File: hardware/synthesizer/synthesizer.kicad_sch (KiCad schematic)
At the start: 5 parts, among them J2 Input 2, J3 Input 1, J4 Output 1, J5 Output 2, J7 RJ45_Abracon_ARJP11A-MASA-B-A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

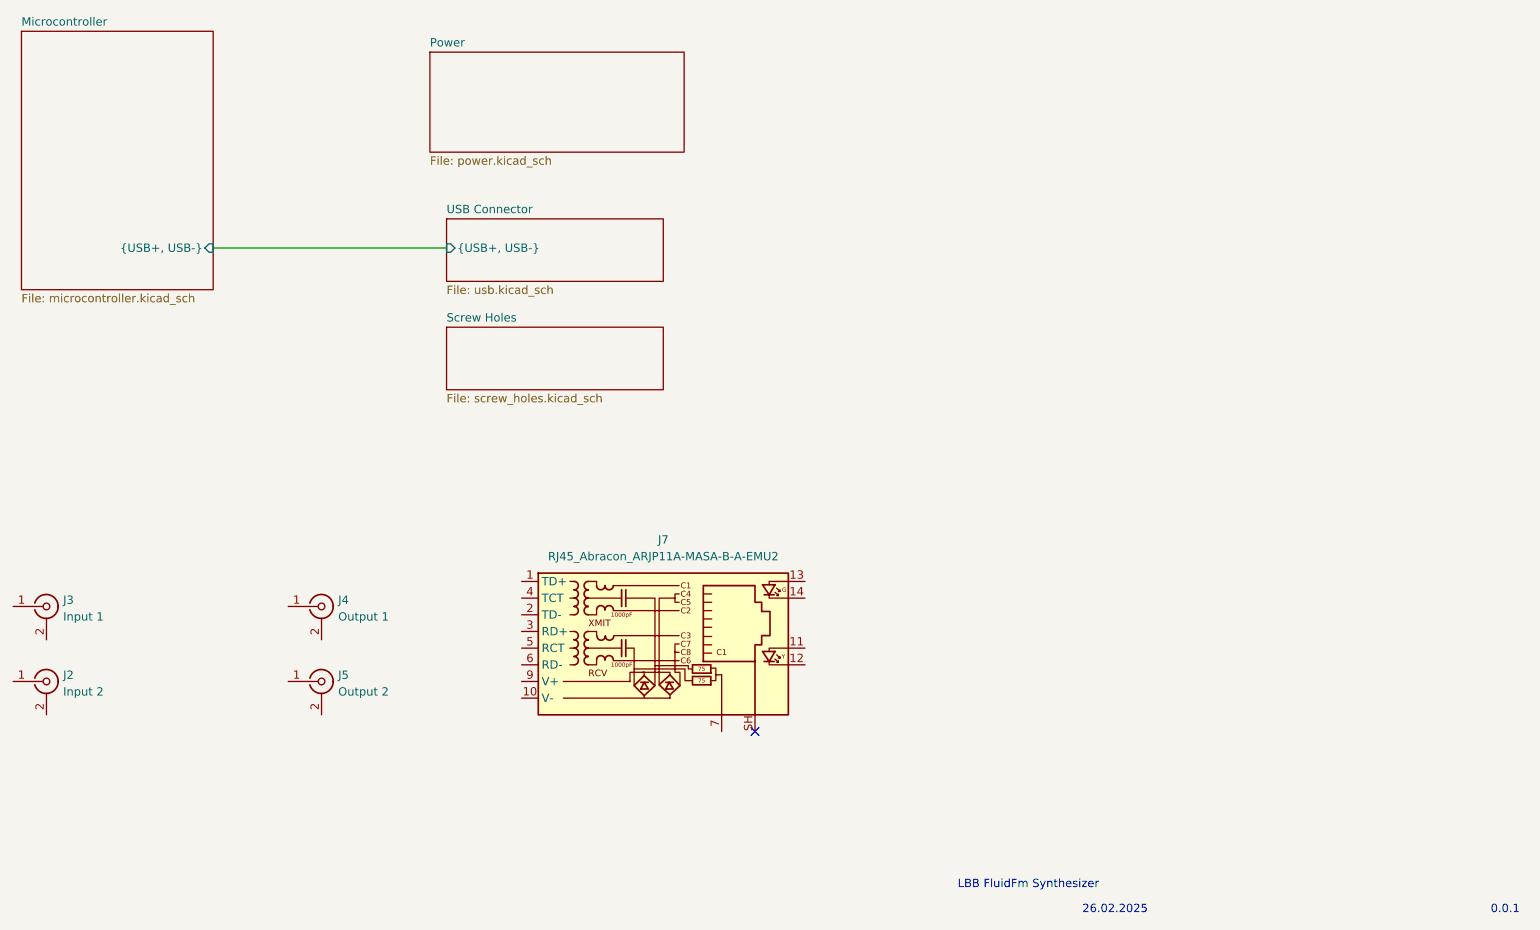
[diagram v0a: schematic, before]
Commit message: work on hardware
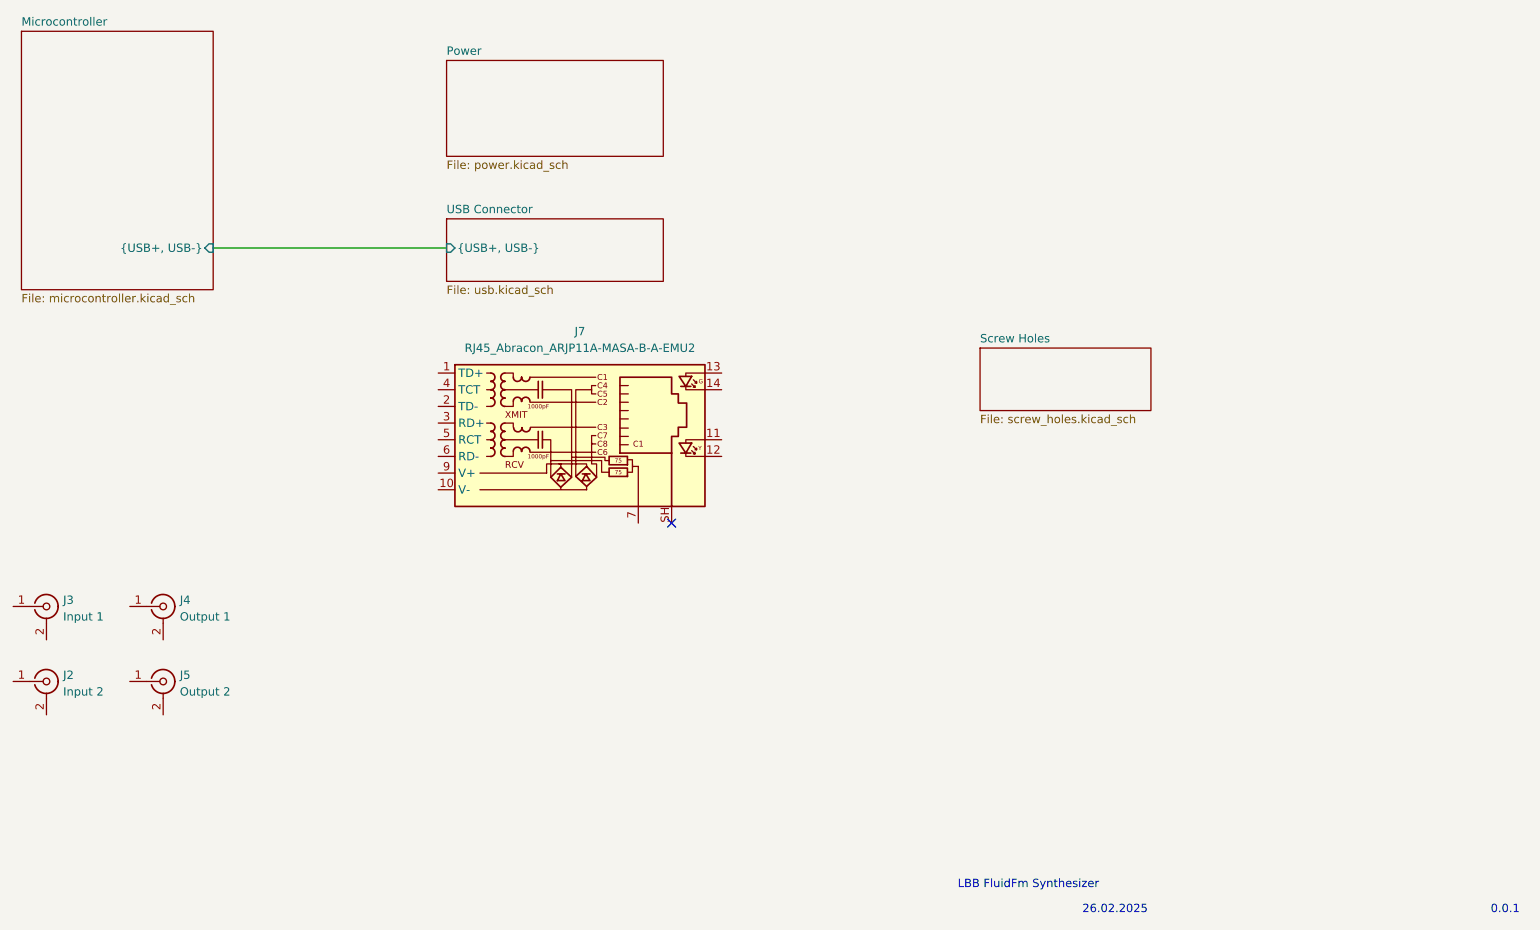
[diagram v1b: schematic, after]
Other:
- moved on the sheet: J4, J5, J7
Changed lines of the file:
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@@
 	)
 	(no_connect
-		(at 157.48 166.37)
+		(at 144.78 134.62)
 	)
 	(wire
@@
 			"AAAAAAAAAAAAAAAAAAAAAAAAAAAAAAAAAAAAAAAAAAAAAAAAAAAAAAAAAAAAAAAAAAAAAAAAAAAA"
 			"AAAAAAAAAAAAAAAAAAAAAAAAAAAAAAAAAAD/AQAAAAAAAAAEAAAAAAAAAAAAAAAAAAAAAAAAAAAA"
+			"AAAAAAAAAAAAAAAAAAAAAAAAAAAAAAAAAAAAAAAAAAAAAAAAAAAAAAAAAAAAAAAAAAAAAAAAAAAA"
+			"AAAAAAAAAAAAAAAAAAAAAAAAAAAAAAAAAAAAAAAAAAAAAAAAAAAAAAAAAAAAAAAAAAAAAAAAAAAA"
+			"AAAAAAAAAAAAAAAAAAAAAAAAAAAAAAAAAAAAAAAAAAAAAAAAAAAAAAAAAAAAAAAAAAAAAAAAAAAA"
+			"AAAAAAAAAAAAAAAAAAAAAAAAAAAAAAAAAAAAAAAAAAAAAAAAAAAAAAAAAAAAAAAAAAAAAAAAAAAA"
+			"AAAAAAAAAAAAAAAAAAAAAAAAAAAAAAAAAAAAAAAAAAAAAAAAAAAAAAAAAAAAAAAAAAAAAAAAAAAA"
+			"AAAAAAAAAAAAAAAAAAAAAAAAAAAAAAAAAAAAAAAAAAAAAAAAAAAAAAAAAAAAAAAAAAAAAAAAAAAA"
+			"AAAAAAAAAAAAAAAAAAAAAAAAAAAAAAAAAAAAAAAAAAAAAAAAAAAAAAAAAAAAAAAAAAAAAAAAAAAA"
+			"AAAAAAAAAAAAAAAAAAAAAAAAAAAAAAAAAAAAAAAAAAAAAAAAAAAAAAAAAAAAAAAAAAAAAAAAAAAA"
+			"AAAAAAAAAAAAAAAAAAAAAAAAAAAAAAAAAAAAAAAAAAAAAAAAAAAAAAAAAAAAAAAAAAAAAAAAAAAA"
+			"AAAAAAAAAAAAAAAAAAAAAAAAAAAAAAAAAAAAAAAAAAAAAAAAAAAAAAAAAAAAAAAAAAAAAAAAAAAA"
+			"AAAAAAAAAAAAAAAAAAAAAAAAAAAAAAAAAAAAAAAAAAAAAAAAAAAAAAAAAAAAAAAAAAAAAAAAAAAA"
+			"AAAAAAAAAAAAAAAAAAAAAAAAAAAAAAAAAAAAAAAAAAAAAAAAAAAAAAAAAAAAAAAAAAAAAAAAAAAA"
+			"AAAAAAAAAAAAAAAAAAAAAAAAAAAAAAAAAAAAAAAAAAAAAAAAAAAAAAAAAAAAAAAAAAAAAAAAAAAA"
+			"AAAAAAAAAAAAAAAAAAAAAAAAAAAAAAAAAAAAAAAAAAAAAAAAAAAAAAAAAAAAAAAAAAAAAAAAAAAA"
+			"AAAAAAAAAAAAAAAAAAAAAAAAAAAAAAAAAAAAAAAAAAAAAAAAAAAAAAAAAAAAAAAAAAAAAAAAAAAA"
+			"AAAAAAAAAAAAAAAAAAAAAAAAAAAAAAAAAAAAAAAAAAAAAAAAAAAAAAAAAAAAAAAAAAAAAAAAAAAA"
+			"AAAAAAAAAAAAAAAAAAAAAAAAAAAAAAAAAAAAAAAAAAAAAAAAAAAAAAAAAAAAAAAAAAAAAAAAAAAA"
+			"AAAAAAAAAAAAAAAAAAAAAAAAAAAAAAAAAAAAAAAAAAAAAAAAAAAAAAAAAAAAAAAAAAAAAAAAAAAA"
 			"AAAAAAAAAAAAAAAAAAAAAAAAAAAAAAAAAAAAAAAAAAAAAAAAAAAAAAAAAAAAAAAAAAAAAAAAAAAA"
 			"AAAAAAAAAAAAAAAAAAAAAAAAAAAAAAAAAAAAAAAAAAAAAAAAAAAAAAAAAAAAAAAAAAAAAAAAAAAA"
@@
 			"AAAAAAAAAAAAAAAAAAAAAAAAAAAAAAAAAAAAAAAAAAAAAAAAAAAAAAAAAAAAAAAAAAAAAAAAAAAA"
 			"AAAAAAAAAAAAAAAAAAAAAAAAAAAAAAAAAAAAAAAAAAAAAAAAAAAAAAAAAAAAAAAAAAAAAAAAAAAA"
-			"AAAAAAAAAA=="
+			"AAAAAAAAAFUEBhMCVVMxEzARBgNVBAgMCkNhbGlmb3JuaWExETAPBgNVBAcMCFNhbiBKb3NlMRYw"
+			"FAYDVQQKDA1BZG9iZSBTeXN0ZW1zMRkwFwYDVQQLDBBDbG91ZCBUZWNobm9sb2d5MSMwIQYDVQQD"
+			"DBpBZG9iZSBJbnRlcm1lZGlhdGUgQ0EgMTAtMzAeFw0xODA4MjAxMzE4NDJaFw0yNTA4MTgxMzE4"
+			"NDJaMIGRMQswCQYDVQQGEwJVUzETMBEGA1UECAwKQ2FsaWZvcm5pYTERMA8GA1UEBwwIU2FuIEpv"
+			"c2UxFjAUBgNVBAoMDUFkb2JlIFN5c3RlbXMxGTAXBgNVBAsMEENsb3VkIFRlY2hub2xvZ3kxJzAl"
+			"BgNVBAMMHkFkb2JlIENvbnRlbnQgQ2VydGlmaWNhdGUgMTAtNTCCAiIwDQYJKoZIhvcNAQEBBQAD"
+			"ggIPADCCAgoCggIBAMtLOHVVhlS/inUWJNxCVZygntoibXj1gsmxvsZhKK73vqmc4bFETqaqvpAz"
+			"2YJFUf+vGgElcAWXikYstRHlzcxEw8QGXwnv45RIztsWmwBNo5W6b0zHlJTZoTwC5LdHGrsnO5JL"
+			"VEWwq+SYWMfRDgmJ5kYqRYwQkQ14qpe0w7r1j2iy2QC/4AHM4/aj/5EDUEj8sHQ0gll30q2i8QRD"
+			"aTTLAdlmQ0m7W477tbZRljs/4a6j9m++O+VCQ7wLobFNtZYTGyrRS5ABMTHyMWkd+Pgew8HiIrsO"
+			"fx2ZfoKOPaJN++QnRA9nOUKnbrhp2MdV2Os2s+pi6sdwI/p61C+qaIV4xYj+LpH9d5tLiiycC4l0"
+			"SXHY53Kr8loUMtrvat6EOb/0nAufHhUDont1cAPbdxnVpJY+M/up4LLGDE64uiDEJBPGf9hRAmcH"
+			"QbW49AFw+wtQpf8UWH1JccTjeiTp/tzXtXjiNQ+72AOEqt86iyQMYxGPWgP5aktS0SLz7GyQggNZ"
+			"GSqW/LWmVUfVNqXLQPgsVAp8KZrnkwCAYFIZFmo5odJCLtXsgr8UK6aYJDTCLnkFwG1dPf20kNm+"
+			"HOCOZmVOiVYKnfqeiseaJ83bhCL+A+B7qiYXiB7s7xAUYaWosZXeoI157+nGkczhKWJmQBHXQCy0"
+			"9UJ7V1HwKdmUnrjBAgMBAAGjIDAeMA4GA1UdDwEB/wQEAwIHgDAMBgNVHRMBAf8EAjAAMA0GCSqG"
+			"SIb3DQEBDQUAA4ICAQCIpEoxHQmM1a/cHooG48XTTaf0CRIeCV53UGt9pH4/gXB23dZr9U57iXhU"
+			"2N8xLdLOICEnH/nTXoK8eiGxW/E3pAzW/nBcab/wd4MIIiYRogcLhAO5DWVYXGiBF9fqBbtGkwLX"
+			"ma71Lj9Mfg=="
 		)
 	)
 	(symbol
 		(lib_id "Connector:RJ45_Abracon_ARJP11A-MASA-B-A-EMU2")
-		(at 142.24 153.67 0)
+		(at 129.54 121.92 0)
 		(unit 1)
 		(exclude_from_sim no)
@@
 		(fields_autoplaced yes)
 		(property "Reference" "J7"
-			(at 143.51 137.16 0)
+			(at 130.81 105.41 0)
 			(effects
 				(font
@@
 		)
 		(property "Value" "RJ45_Abracon_ARJP11A-MASA-B-A-EMU2"
-			(at 143.51 139.7 0)
+			(at 130.81 107.95 0)
 			(effects
 				(font
@@
 		)
 		(property "Footprint" "Connector_RJ:RJ45_Abracon_ARJP11A-MA_Horizontal"
-			(at 142.24 138.43 0)
+			(at 129.54 106.68 0)
 			(effects
 				(font
@@
 		)
 		(property "Datasheet" "https://abracon.com/Magnetics/lan/ARJP11A.PDF"
-			(at 142.24 135.89 0)
+			(at 129.54 104.14 0)
 			(effects
 				(font
@@
 		)
 		(property "Description" "RJ45 PoE 10/100 Base-TX Jack with Magnetic Module"
-			(at 142.24 153.67 0)
+			(at 129.54 121.92 0)
 			(effects
 				(font
@@
 	(symbol
 		(lib_id "Connector:Conn_Coaxial")
-		(at 91.44 147.32 0)
+		(at 67.31 147.32 0)
 		(unit 1)
 		(exclude_from_sim no)
@@
 		(fields_autoplaced yes)
 		(property "Reference" "J4"
-			(at 93.98 146.3431 0)
+			(at 69.85 146.3431 0)
 			(effects
 				(font
@@
 		)
 		(property "Value" "Output 1"
-			(at 93.98 148.8831 0)
+			(at 69.85 148.8831 0)
 			(effects
 				(font
@@
 		)
 		(property "Footprint" "Connector_Coaxial:BNC_TEConnectivity_1478035_Horizontal"
-			(at 91.44 147.32 0)
+			(at 67.31 147.32 0)
 			(effects
 				(font
@@
 		)
 		(property "Datasheet" "~"
-			(at 91.44 147.32 0)
+			(at 67.31 147.32 0)
 			(effects
 				(font
@@
 		)
 		(property "Description" "coaxial connector (BNC, SMA, SMB, SMC, Cinch/RCA, LEMO, ...)"
-			(at 91.44 147.32 0)
+			(at 67.31 147.32 0)
 			(effects
 				(font
@@
 	(symbol
 		(lib_id "Connector:Conn_Coaxial")
-		(at 91.44 158.75 0)
+		(at 67.31 158.75 0)
 		(unit 1)
 		(exclude_from_sim no)
@@
 		(fields_autoplaced yes)
 		(property "Reference" "J5"
-			(at 93.98 157.7731 0)
+			(at 69.85 157.7731 0)
 			(effects
 				(font
@@
 		)
 		(property "Value" "Output 2"
-			(at 93.98 160.3131 0)
+			(at 69.85 160.3131 0)
 			(effects
 				(font
@@
 		)
 		(property "Footprint" "Connector_Coaxial:BNC_TEConnectivity_1478035_Horizontal"
-			(at 91.44 158.75 0)
+			(at 67.31 158.75 0)
 			(effects
 				(font
@@
 		)
 		(property "Datasheet" "~"
-			(at 91.44 158.75 0)
+			(at 67.31 158.75 0)
 			(effects
 				(font
@@
 		)
 		(property "Description" "coaxial connector (BNC, SMA, SMB, SMC, Cinch/RCA, LEMO, ...)"
-			(at 91.44 158.75 0)
+			(at 67.31 158.75 0)
 			(effects
 				(font
@@
 	)
 	(sheet
-		(at 107.95 62.865)
-		(size 38.735 15.24)
+		(at 110.49 64.135)
+		(size 33.02 14.605)
 		(exclude_from_sim no)
 		(in_bom yes)
@@
 		)
 		(property "Sheetname" "Power"
-			(at 107.95 62.1534 0)
+			(at 110.49 63.4234 0)
 			(effects
 				(font
@@
 		)
 		(property "Sheetfile" "power.kicad_sch"
-			(at 107.95 78.6896 0)
+			(at 110.49 79.3246 0)
 			(effects
 				(font
@@
 	)
 	(sheet
-		(at 110.49 104.775)
-		(size 33.02 9.525)
+		(at 191.77 107.95)
+		(size 26.035 9.525)
 		(exclude_from_sim no)
 		(in_bom yes)
@@
 		)
 		(property "Sheetname" "Screw Holes"
-			(at 110.49 104.0634 0)
+			(at 191.77 107.2384 0)
 			(effects
 				(font
@@
 		)
 		(property "Sheetfile" "screw_holes.kicad_sch"
-			(at 110.49 114.8846 0)
-			(effects
-				(font
+			(at 191.77 118.0596 0)
+			(effects
+				(font
